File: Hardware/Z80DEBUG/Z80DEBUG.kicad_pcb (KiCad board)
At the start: 2 copper layers, 105 x 53 mm, 50 parts, among them J1 Conn_02x40_Odd_Even, U1 74HC373, U2 74HC373, U3 74HC373, U4 74HC373

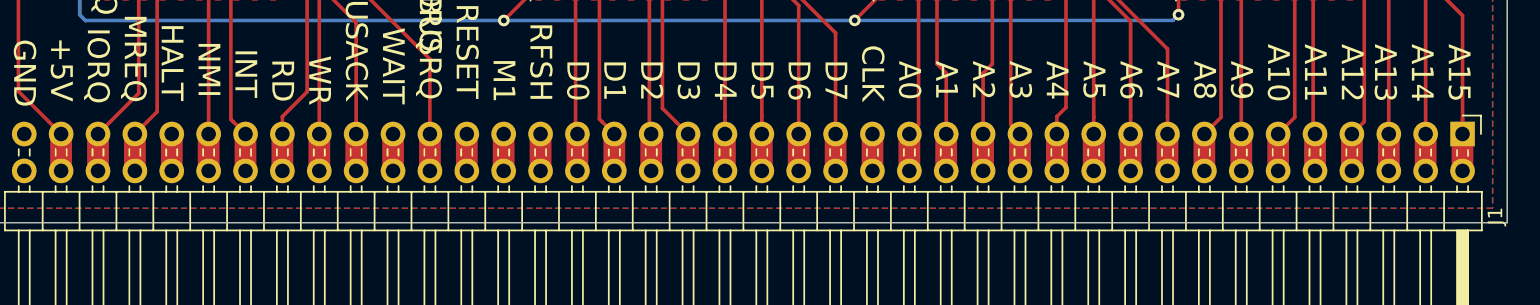
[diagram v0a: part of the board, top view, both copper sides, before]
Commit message: debug fix
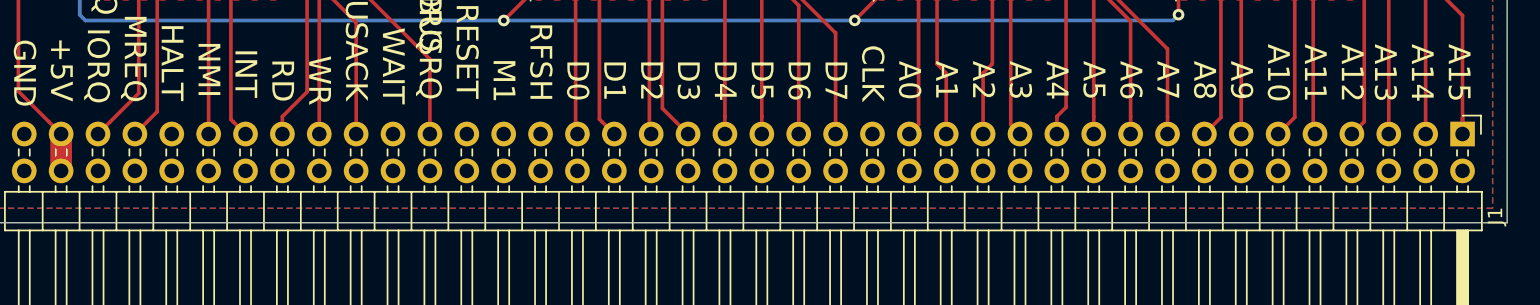
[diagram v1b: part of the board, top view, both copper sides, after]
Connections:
- J1 pad 10: /A11 -> Net-(J1-Pad10)
- J1 pad 12: /A10 -> Net-(J1-Pad12)
- J1 pad 14: /A9 -> Net-(J1-Pad14)
- J1 pad 16: /A8 -> Net-(J1-Pad16)
- J1 pad 18: /A7 -> Net-(J1-Pad18)
- J1 pad 2: /A15 -> Net-(J1-Pad2)
- J1 pad 20: /A6 -> Net-(J1-Pad20)
- J1 pad 22: /A5 -> Net-(J1-Pad22)
- J1 pad 24: /A4 -> Net-(J1-Pad24)
- J1 pad 26: /A3 -> Net-(J1-Pad26)
- J1 pad 28: /A2 -> Net-(J1-Pad28)
- J1 pad 30: /A1 -> Net-(J1-Pad30)
- J1 pad 32: /A0 -> Net-(J1-Pad32)
- J1 pad 34: /CLK -> Net-(J1-Pad34)
- J1 pad 36: /D7 -> Net-(J1-Pad36)
- J1 pad 38: /D6 -> Net-(J1-Pad38)
- J1 pad 4: /A14 -> Net-(J1-Pad4)
- J1 pad 40: /D5 -> Net-(J1-Pad40)
- J1 pad 42: /D4 -> Net-(J1-Pad42)
- J1 pad 44: /D3 -> Net-(J1-Pad44)
- J1 pad 46: /D2 -> Net-(J1-Pad46)
- J1 pad 48: /D1 -> Net-(J1-Pad48)
- J1 pad 50: /D0 -> Net-(J1-Pad50)
- J1 pad 52: /RFSH -> Net-(J1-Pad52)
- J1 pad 54: /M1 -> Net-(J1-Pad54)
- J1 pad 56: /RESET -> Net-(J1-Pad56)
- J1 pad 58: /BUSRQ -> Net-(J1-Pad58)
- J1 pad 6: /A13 -> Net-(J1-Pad6)
- J1 pad 60: /WAIT -> Net-(J1-Pad60)
- J1 pad 62: /BUSACK -> Net-(J1-Pad62)
- J1 pad 64: /WR -> Net-(J1-Pad64)
- J1 pad 66: /RD -> Net-(J1-Pad66)
- J1 pad 68: /INT -> Net-(J1-Pad68)
- J1 pad 70: /NMI -> Net-(J1-Pad70)
- J1 pad 72: /HALT -> Net-(J1-Pad72)
- J1 pad 74: /MREQ -> Net-(J1-Pad74)
- J1 pad 76: /IORQ -> Net-(J1-Pad76)
- J1 pad 8: /A12 -> Net-(J1-Pad8)
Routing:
- net /MREQ: track 13.5 -> 11.0 mm
- net /WR: track 27.7 -> 25.1 mm
- net /WAIT: track 2.54 -> 0.00 mm
- net /RFSH: track 2.54 -> 0.00 mm
- net /RESET: track 2.54 -> 0.00 mm
- net /RD: track 29.3 -> 26.7 mm
- net /NMI: track 13.0 -> 10.5 mm
- net /M1: track 2.54 -> 0.00 mm
- net /IORQ: track 14.1 -> 11.5 mm
- net /INT: track 13.3 -> 10.8 mm
- net /HALT: track 2.54 -> 0.00 mm
- net /D7: track 26.8 -> 24.3 mm
- net /D6: track 26.4 -> 23.8 mm
- net /D5: track 29.2 -> 26.7 mm
- net /D4: track 29.2 -> 26.6 mm
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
